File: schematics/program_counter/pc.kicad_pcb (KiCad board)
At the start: 2 copper layers, 100 x 91 mm, 18 parts, among them U1 74HC00, U2 74HC193, U3 74HC193, U4 74HC193, U5 74HC193, U6 74HC245, U7 74HC245

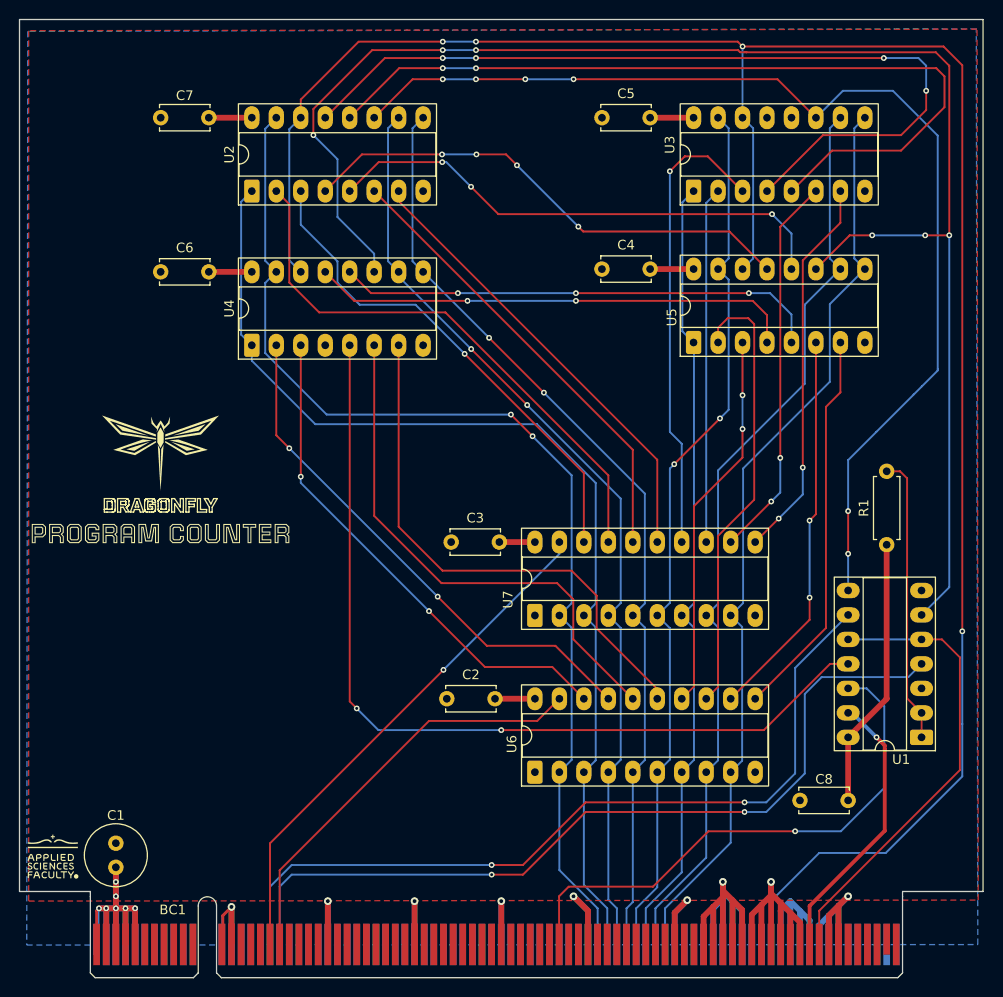
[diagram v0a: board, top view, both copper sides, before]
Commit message: fix(pc)
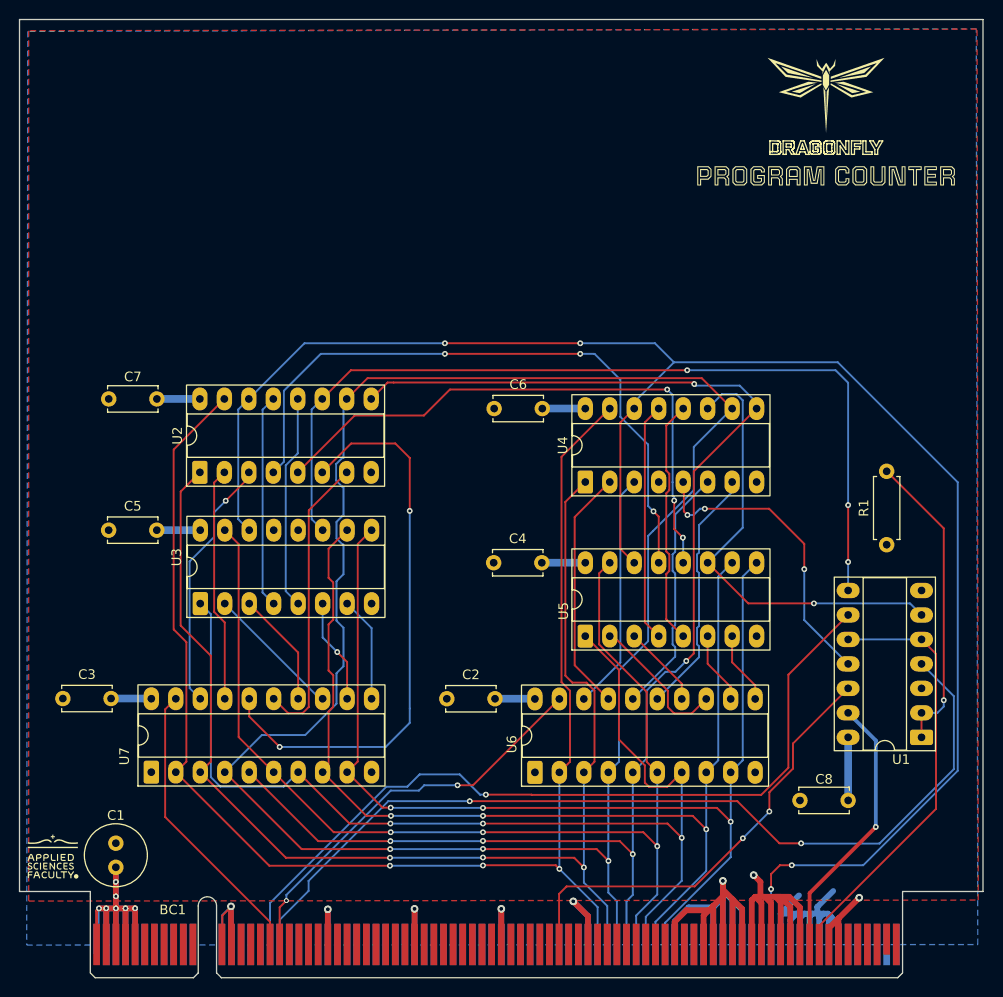
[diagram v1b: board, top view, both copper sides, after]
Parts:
- moved kibuzzard-6911BE41 78.4 mm to (190.2, 50.2)
- moved C5 66.7 mm to (115.8, 87.0)
- moved U3 66.7 mm to (125.3, 94.6)
- moved C3 43.4 mm to (111.0, 104.5)
- moved U7 43.0 mm to (120.2, 112.1)
- moved C6 37.4 mm to (155.8, 74.4)
- moved U4 37.4 mm to (165.2, 82.0)
- moved U5 32.5 mm to (165.2, 98.0)
- moved C4 32.5 mm to (155.7, 90.4)
- moved U2 29.7 mm to (125.2, 81.0)
- moved C7 29.7 mm to (120.8, 73.4)
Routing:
- net /Pl: track 162.2 -> 47.3 mm, vias 6 -> 1
- net /DATA2: track 98.2 -> 195.9 mm, vias 2 -> 3
- net Net-(U2-~{BO}): track 90.0 -> 22.2 mm, vias 4 -> 0
- net Net-(U2-~{CO}): track 86.9 -> 22.3 mm, vias 2 -> 0
- net /CPu: track 92.8 -> 31.9 mm, vias 2 -> 3
- net /DATA3: track 98.1 -> 147.4 mm, vias 2 -> 5
- net /RESET: track 218.7 -> 181.3 mm
- net /DH4: track 48.7 -> 12.0 mm, vias 1 -> 0
- net /DH1: track 58.4 -> 24.4 mm
- net /DL7: track 40.6 -> 7.51 mm
- net /DL6: track 40.6 -> 7.51 mm, vias 2 -> 0
- net /DL5: track 46.9 -> 15.0 mm
- net /DATA0: track 114.8 -> 146.1 mm, vias 2 -> 3
- net /DL4: track 39.6 -> 8.56 mm, vias 2 -> 0
- net /DATA5: track 82.3 -> 113.0 mm, vias 0 -> 3
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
